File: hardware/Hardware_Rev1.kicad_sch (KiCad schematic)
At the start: 160 parts, among them J1 RJ45_LED_Shielded, J2 6P6C, Q1 BSS138, Q10 AO3401A, Q11 AO3401A, Q12 AO3401A, Q13 BSS138, Q14 BSS138, Q15 BSS138, Q16 AO3401A, Q17 AO3401A, Q18 AO3401A, Q19 BSS138, Q2 BSS138, Q20 BSS138, Q21 BSS138, Q22 AO3401A, Q23 AO3401A, Q24 AO3401A, Q3 BSS138, Q4 AO3401A, Q5 AO3401A, Q6 AO3401A, Q7 BSS138, Q8 BSS138, Q9 BSS138, U1 OKI, U2 Teensy4.1_DEV-16771

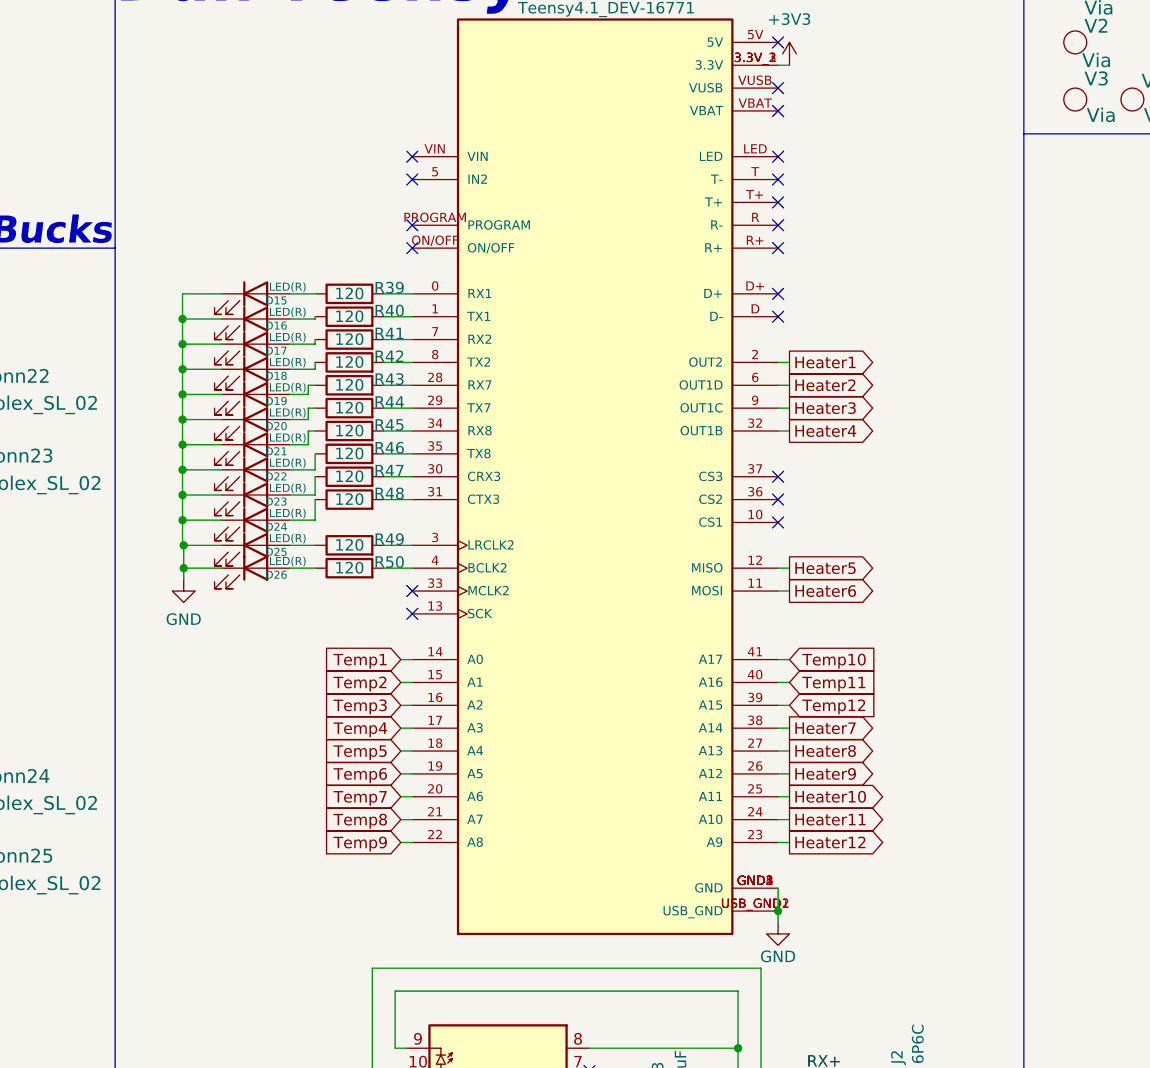
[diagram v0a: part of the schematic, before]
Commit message: Cleaned traces
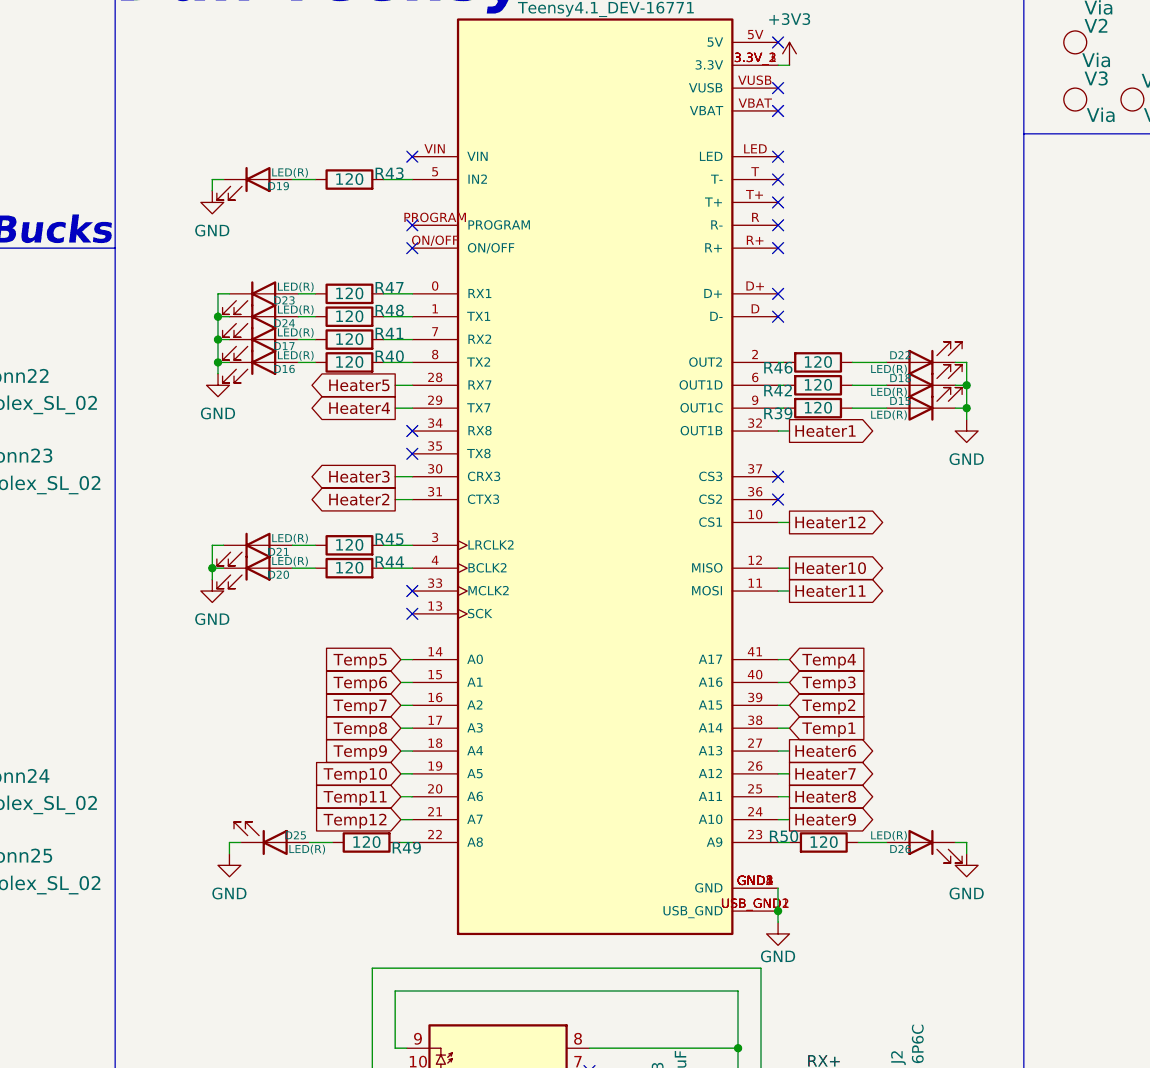
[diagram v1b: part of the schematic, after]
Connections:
- net Heater1: now also U2.32 (OUT1B); no longer U2.2 (OUT2)
- net Heater10: now also U2.12 (MISO); no longer U2.25 (A11)
- net Heater11: now also U2.11 (MOSI); no longer U2.24 (A10)
- net Heater12: now also U2.10 (CS1); no longer U2.23 (A9)
- net Heater2: now also U2.31 (CTX3); no longer U2.6 (OUT1D)
- net Heater3: now also U2.30 (CRX3); no longer U2.9 (OUT1C)
- net Heater4: now also U2.29 (TX7); no longer U2.32 (OUT1B)
- net Heater5: now also U2.28 (RX7); no longer U2.12 (MISO)
- net Heater6: now also U2.27 (A13); no longer U2.11 (MOSI)
- net Heater7: now also U2.26 (A12); no longer U2.38 (A14)
- net Heater8: now also U2.25 (A11); no longer U2.27 (A13)
- net Heater9: now also U2.24 (A10); no longer U2.26 (A12)
- net Temp1: now also U2.38 (A14); no longer U2.14 (A0)
- net Temp10: now also U2.19 (A5); no longer U2.41 (A17)
- net Temp11: now also U2.20 (A6); no longer U2.40 (A16)
- net Temp12: now also U2.21 (A7); no longer U2.39 (A15)
- net Temp2: now also U2.39 (A15); no longer U2.15 (A1)
- net Temp3: now also U2.40 (A16); no longer U2.16 (A2)
- net Temp4: now also U2.41 (A17); no longer U2.17 (A3)
- net Temp5: now also U2.14 (A0); no longer U2.18 (A4)
- net Temp6: now also U2.15 (A1); no longer U2.19 (A5)
- net Temp7: now also U2.16 (A2); no longer U2.20 (A6)
- net Temp8: now also U2.17 (A3); no longer U2.21 (A7)
- net Temp9: now also U2.18 (A4); no longer U2.22 (A8)
- net at R40.2: now also U2.8 (TX2); no longer U2.1 (TX1)
- net at U2.0 (RX1): now also R47.2; no longer R39.2
- net at R43.2: now also U2.5 (IN2); no longer U2.28 (RX7)
- net at R44.2: now also U2.4 (BCLK2); no longer U2.29 (TX7)
- net at R49.2: now also U2.22 (A8); no longer U2.3 (LRCLK2)
- net at R48.2: now also U2.1 (TX1); no longer U2.31 (CTX3)
- net at R45.2: now also U2.3 (LRCLK2); no longer U2.34 (RX8)
- net at R46.2: now also U2.2 (OUT2); no longer U2.35 (TX8)
- net at R50.2: now also U2.23 (A9); no longer U2.4 (BCLK2)
- net at R42.2: now also U2.6 (OUT1D); no longer U2.8 (TX2)
- new net: R39.2, U2.9 (OUT1C)
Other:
- moved on the sheet: D15, D16, D17, D18, D19, D20, D21, D22, D23, D24, D25, D26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
